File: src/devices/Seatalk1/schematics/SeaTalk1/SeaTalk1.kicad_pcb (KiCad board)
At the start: 2 copper layers, 56 x 65 mm, 24 parts, among them J1 Raspberry_Pi_2_3, J3 Conn_01x03_Pin, Q1 BC557, Q2 BC547, Q3 BC547, Q4 BC547, Q5 BC547, Q6 BC547

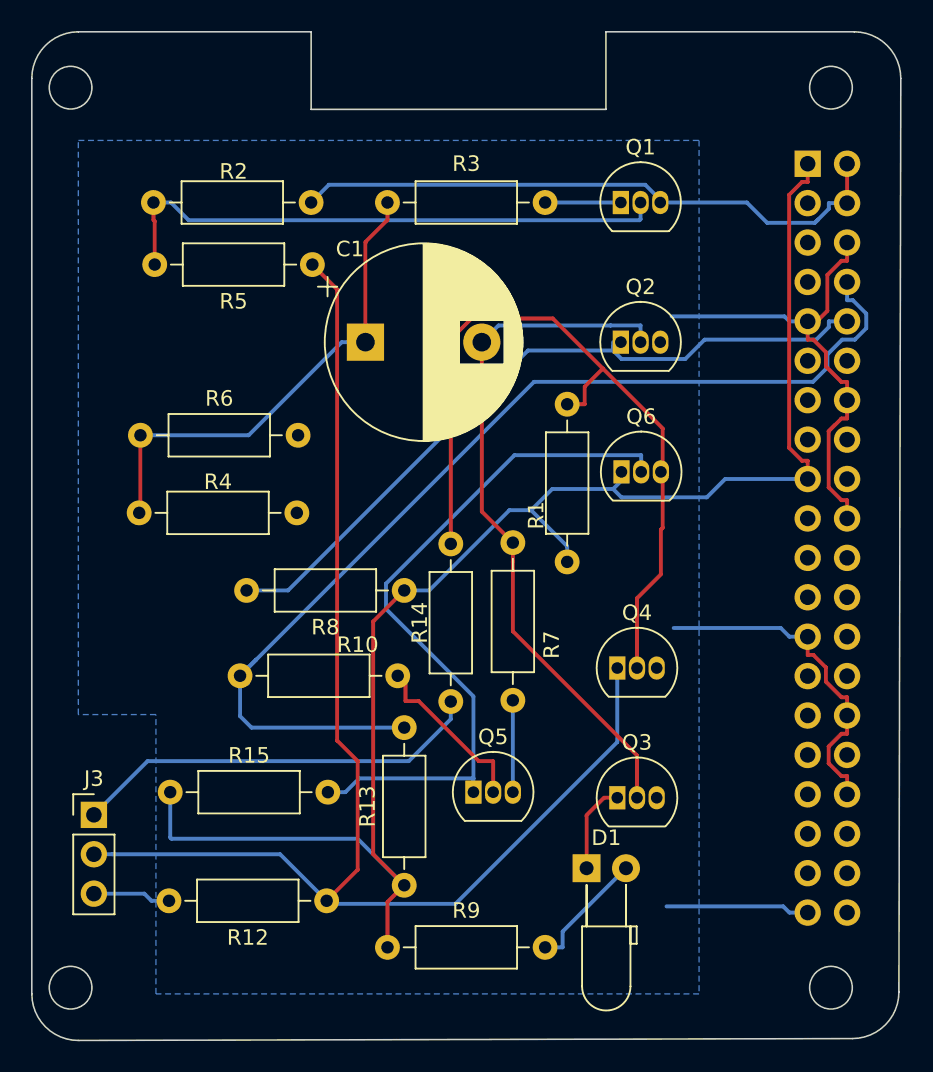
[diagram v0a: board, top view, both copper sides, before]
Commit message: Documentation started
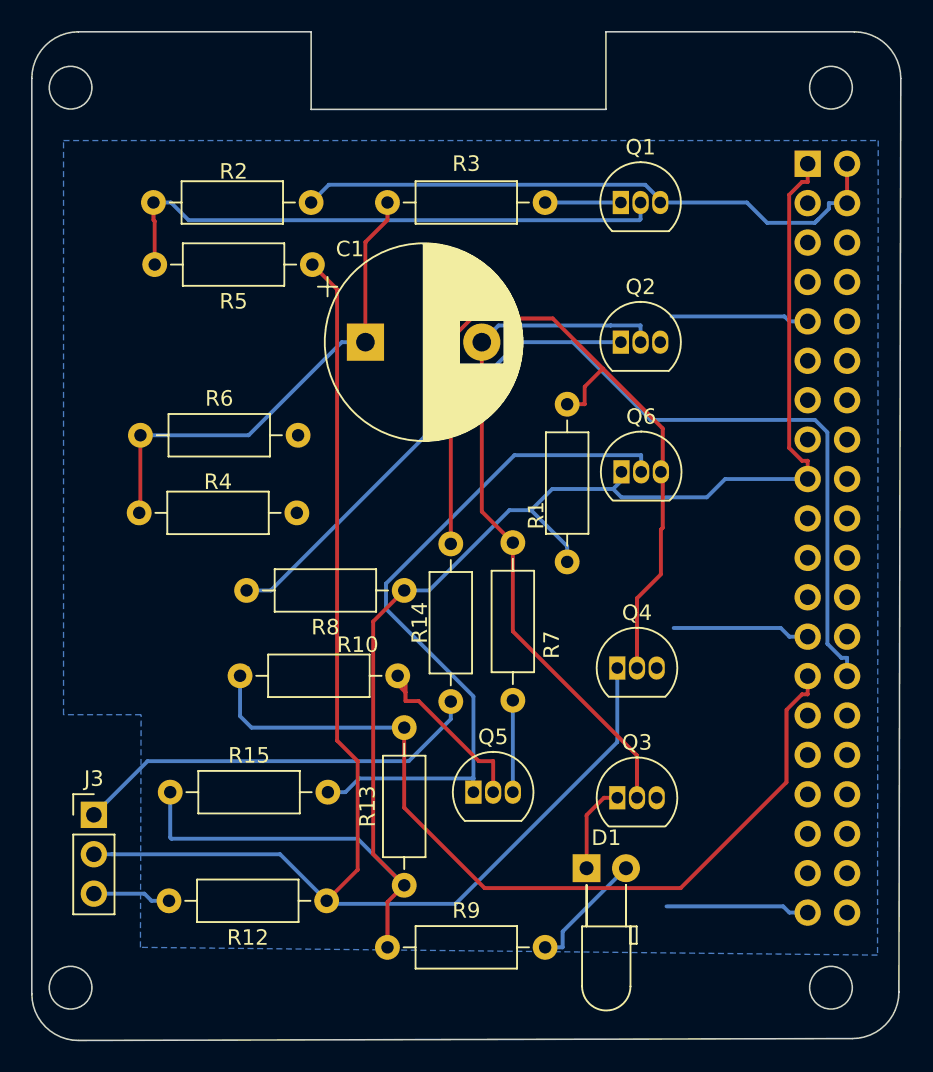
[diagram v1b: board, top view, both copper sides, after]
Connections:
- J1 pad 10: Net-(J1-GPIO15/RXD) -> unconnected-(J1-GPIO15/RXD-Pad10)
- J1 pad 27: unconnected-(J1-ID_SD/GPIO0-Pad27) -> TXD
- J1 pad 28: unconnected-(J1-ID_SC/GPIO1-Pad28) -> Net-(J1-ID_SC/GPIO1)
- J1 pad 8: TXD -> unconnected-(J1-GPIO14/TXD-Pad8)
- Q2 pad 1: Net-(J1-GPIO15/RXD) -> Net-(J1-ID_SC/GPIO1)
- R8 pad 2: Net-(J1-GPIO15/RXD) -> Net-(J1-ID_SC/GPIO1)
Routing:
- net Net-(J1-ID_SC/GPIO1): track 0.00 -> 66.0 mm
- net Net-(J1-GPIO15/RXD): track 47.7 -> 0.00 mm
- net GND: track 95.3 -> 60.3 mm
- net TXD: track 69.1 -> 57.6 mm
- net Net-(Q5-B): track 10.4 -> 11.7 mm
